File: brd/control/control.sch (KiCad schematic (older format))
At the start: 50 parts, among them P1 POWER, P2 PSU, P3 DISPLAY, P4 RS485, P5 PROBE, P6 OUTS, Q1 IRLML2060, Q2 IRLML2060, Q3 IRLML2060, Q4 IRLML2060, Q5 IRLML2060, U1 ATMEGA328-A, U2 25LC1024, U3 MAX13487, U4 MAX13487, X1 16MHz

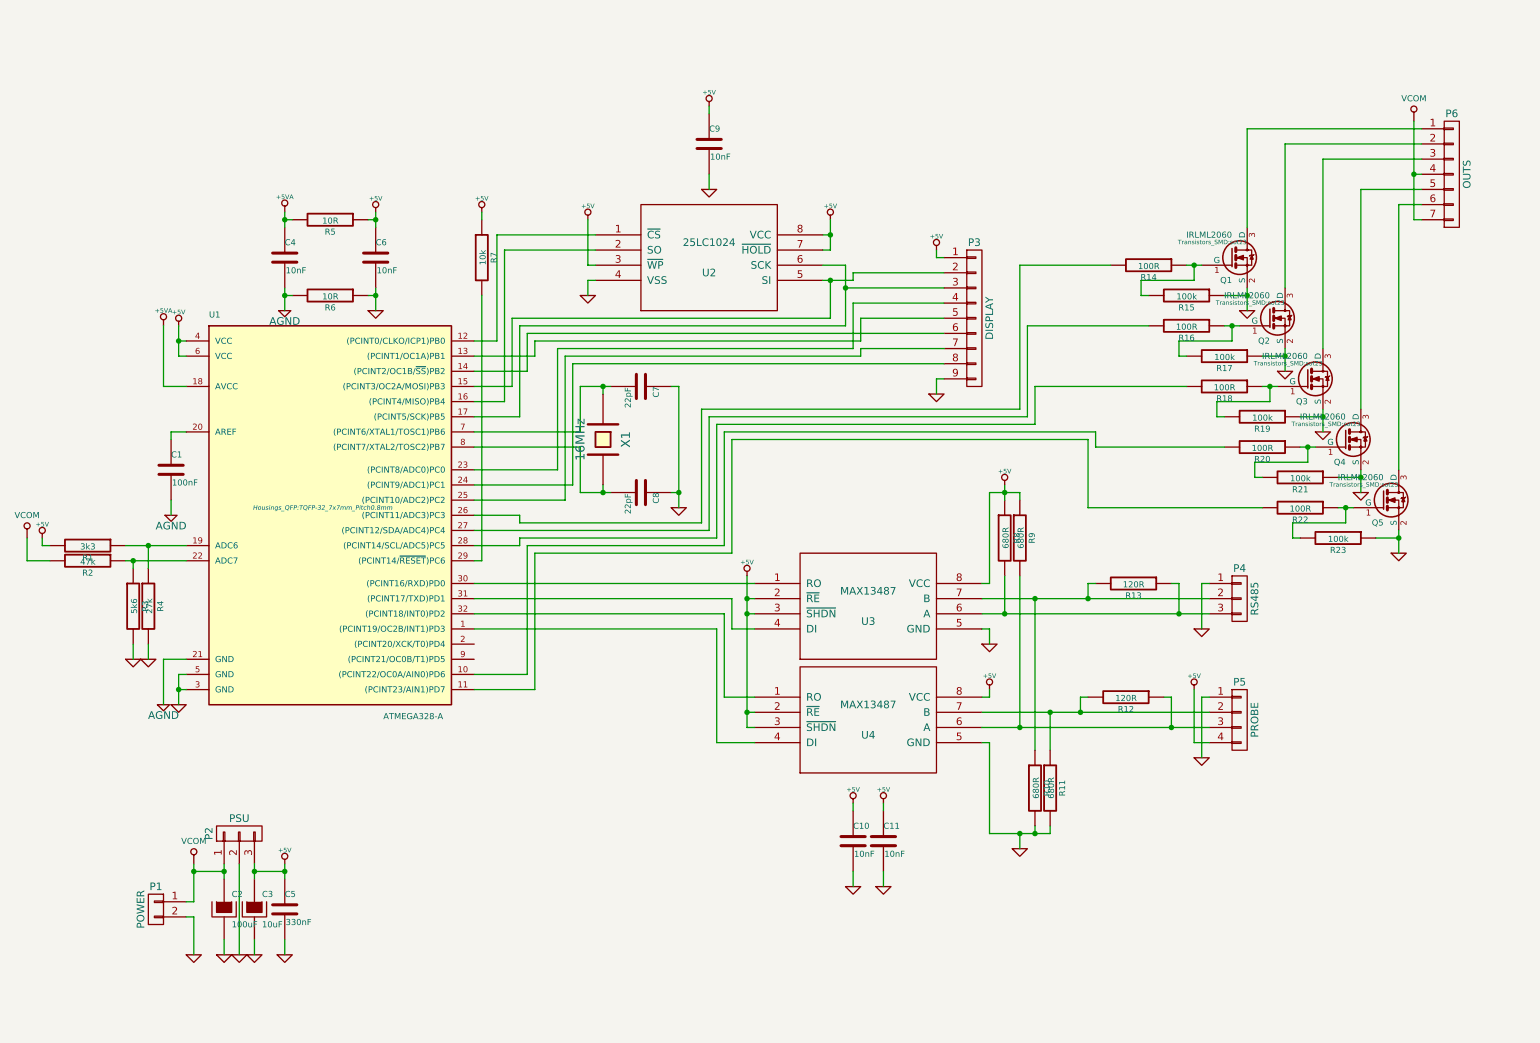
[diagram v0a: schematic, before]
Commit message: chg: dev: backup !wip
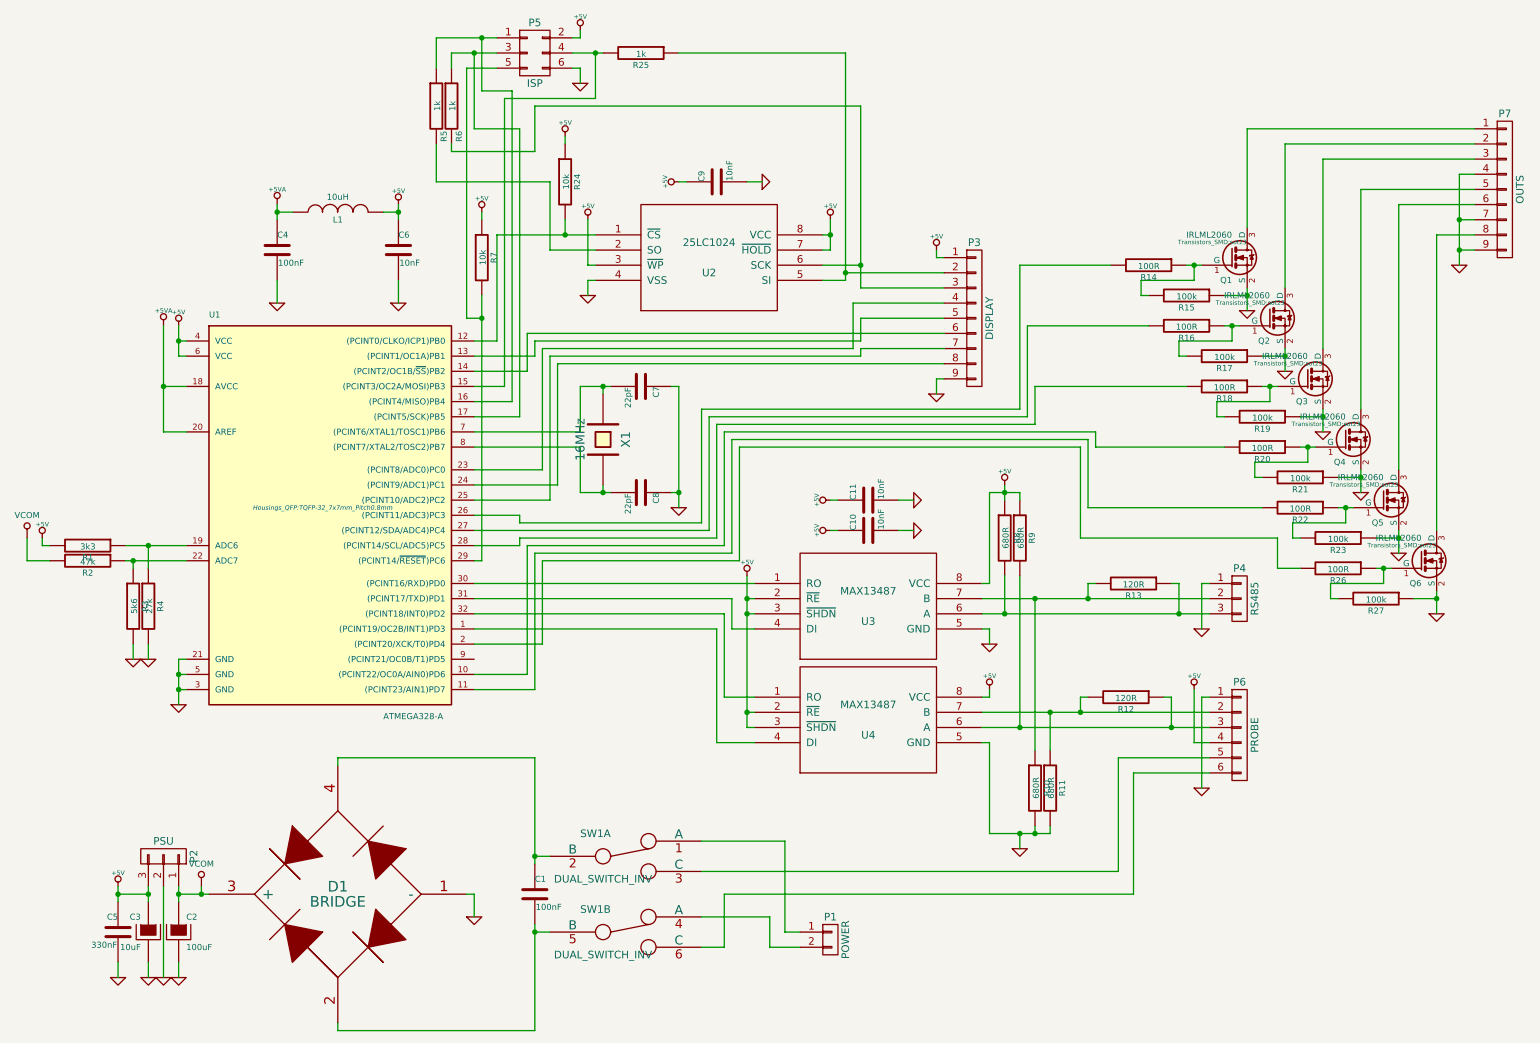
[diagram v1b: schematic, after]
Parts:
- removed P5: PROBE, Sockets_MOLEX_KK-System:Socket_MOLEX-KK-RM2-54mm_Lock_4pin_straight, symbol CONN_01X04
- removed P6: OUTS, symbol CONN_01X07
- added D1: BRIDGE, symbol BRIDGE
- added L1: 10uH, symbol INDUCTOR
- added P5: ISP, symbol CONN_02X03
- added P6: PROBE, symbol CONN_01X06
- added P7: OUTS, symbol CONN_01X09
- added Q6: IRLML2060, Transistors_SMD:sot23, symbol BSS138
- added R24: 10k, symbol R
- added R25: 1k, symbol R
- added R26: 100R, Resistors_SMD:R_0805_HandSoldering, symbol R
- added R27: 100k, Resistors_SMD:R_0805_HandSoldering, symbol R
- added SW1: DUAL_SWITCH_INV, symbol DUAL_SWITCH_INV
- C1: footprint Capacitors_SMD:C_0805_HandSoldering -> (none)
- C4: value 10nF -> 100nF
- R5, R6: value 10R -> 1k; footprint Resistors_SMD:R_0805_HandSoldering -> (none)
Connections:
- net +5V: now also L1.2, P5.2 (P2), P6.4 (P4), R24.1; no longer R5.1
- net +5VA: now also U1.20 (AREF), L1.1; no longer R5.2
- net GND: now also C4.2, U1.21 (GND), D1.1 (-), P5.6 (P6), P6.1 (P1), P7.4 (P4), P7.7 (P7), P7.9 (P9), Q6.2 (S), R27.1; no longer P1.2 (P2), R6.1
- net VCOM: now also D1.3 (+); no longer P1.1 (P1)
- net at U1.12 ((PCINT0/CLKO/ICP1)PB0), U2.1 (~CS): now also R24.2
- net at P3.2 (P2), U2.5 (SI): now also R25.1; no longer U1.15 ((PCINT3/OC2A/MOSI)PB3)
- net at U1.16 ((PCINT4/MISO)PB4): now also R5.1, P5.1 (P1); no longer U2.2 (SO)
- net at P3.3 (P3), U2.6 (SCK): now also R6.2; no longer U1.17 ((PCINT5/SCK)PB5)
- net at U1.2 ((PCINT20/XCK/T0)PD4): now also R26.2
- net at C1.1: now also D1.4, SW1.2 (B); no longer U1.20 (AREF)
- net at R7.2, U1.29 ((PCINT14/~RESET~)PC6): now also P5.5 (P5)
- net at R12.1, R9.2, U4.6 (A): now also P6.3 (P3)
- net at R11.1, R12.2, U4.7 (B): now also P6.2 (P2)
- net at Q1.3 (D): now also P7.1 (P1)
- net at Q2.3 (D): now also P7.2 (P2)
- net at Q3.3 (D): now also P7.3 (P3)
- net at Q4.3 (D): now also P7.5 (P5)
- net at Q5.3 (D): now also P7.6 (P6)
- removed net AGND: C1.2, C4.2, R6.2, U1.21 (GND)
- new net: P5.4 (P4), R25.2, U1.15 ((PCINT3/OC2A/MOSI)PB3)
- new net: P5.3 (P3), R6.1, U1.17 ((PCINT5/SCK)PB5)
- new net: R5.2, U2.2 (SO)
- new net: P1.1 (P1), SW1.1 (A)
- new net: P1.2 (P2), SW1.4 (A)
- new net: Q6.1 (G), R26.1, R27.2
- new net: P7.8 (P8), Q6.3 (D)
- new net: P6.5 (P5), SW1.3 (C)
- new net: P6.6 (P6), SW1.6 (C)
- new net: C1.2, D1.2, SW1.5 (B)
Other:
- moved on the sheet: C10, C11, C2, C3, C4, C5, C6, C9, P1, P2
